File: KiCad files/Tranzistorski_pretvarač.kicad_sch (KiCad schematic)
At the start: 30 parts, among them J1 Screw_Terminal_01x02, J2 Screw_Terminal_01x02, J3 Conn_01x03_Male, J4 Conn_01x01_Male, J5 Screw_Terminal_01x03, J6 Conn_01x01_Male, J7 Conn_01x01_Male, J8 Conn_01x01_Male, Q1 IRLZ44N, U1 SG3524, U2 PC817

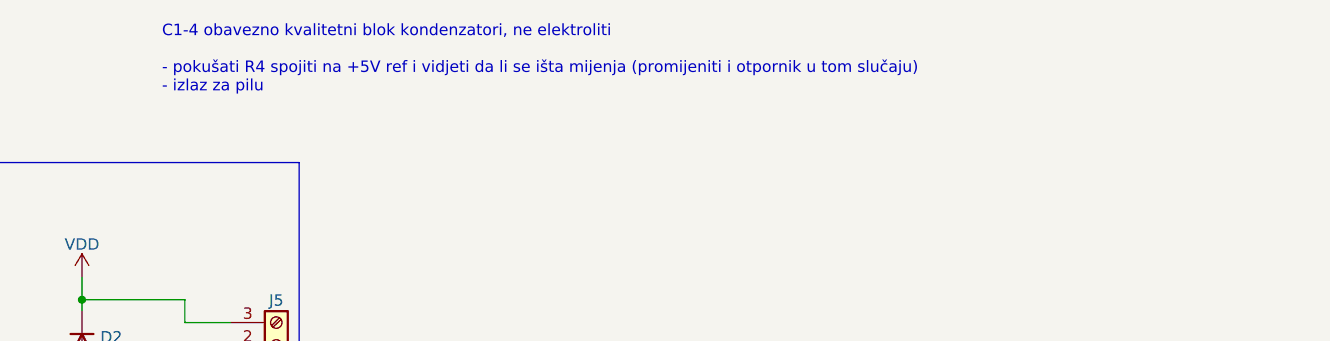
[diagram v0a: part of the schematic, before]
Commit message: notes
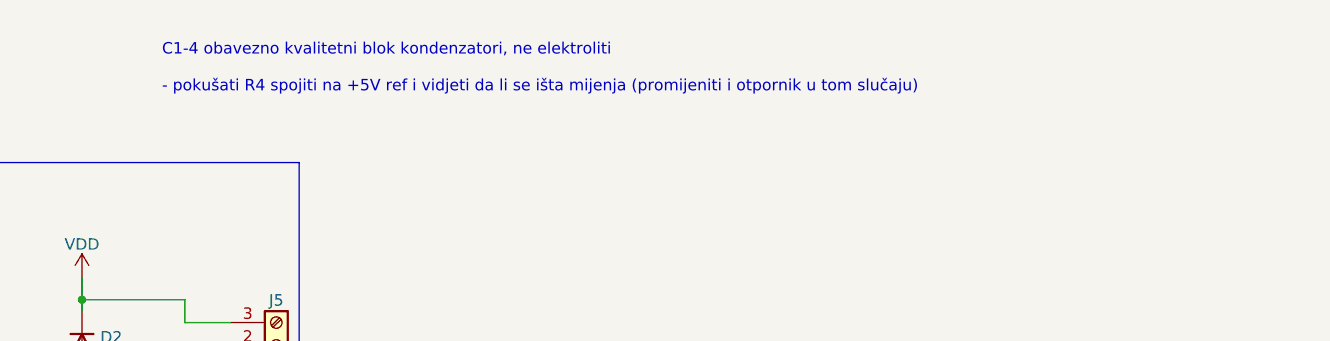
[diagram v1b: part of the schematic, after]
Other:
- note added: "C1-4 obavezno kvalitetni blok kondenzatori, ne elektroliti - pokušati R4 spojiti na +5V ref i vidjeti da li se išta mijenja (promijeniti i otpornik u tom slučaju)"
- note removed: "C1-4 obavezno kvalitetni blok kondenzatori, ne elektroliti - pokušati R4 spojiti na +5V ref i vidjeti da li se išta mijenja (promijeniti i otpornik u tom slučaju) - izlaz za pilu"
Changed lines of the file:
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@@
     (effects (font (size 3 3) (thickness 0.6) bold) (justify left bottom))
   )
-  (text "C1-4 obavezno kvalitetni blok kondenzatori, ne elektroliti\n\n- pokušati R4 spojiti na +5V ref i vidjeti da li se išta mijenja (promijeniti i otpornik u tom slučaju)\n- izlaz za pilu"
+  (text "C1-4 obavezno kvalitetni blok kondenzatori, ne elektroliti\n\n- pokušati R4 spojiti na +5V ref i vidjeti da li se išta mijenja (promijeniti i otpornik u tom slučaju)"
     (at 179.07 27.94 0)
     (effects (font (size 1.27 1.27)) (justify left bottom))
